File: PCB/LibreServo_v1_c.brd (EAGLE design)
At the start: 52.5 x 61.8 mm, 192 parts

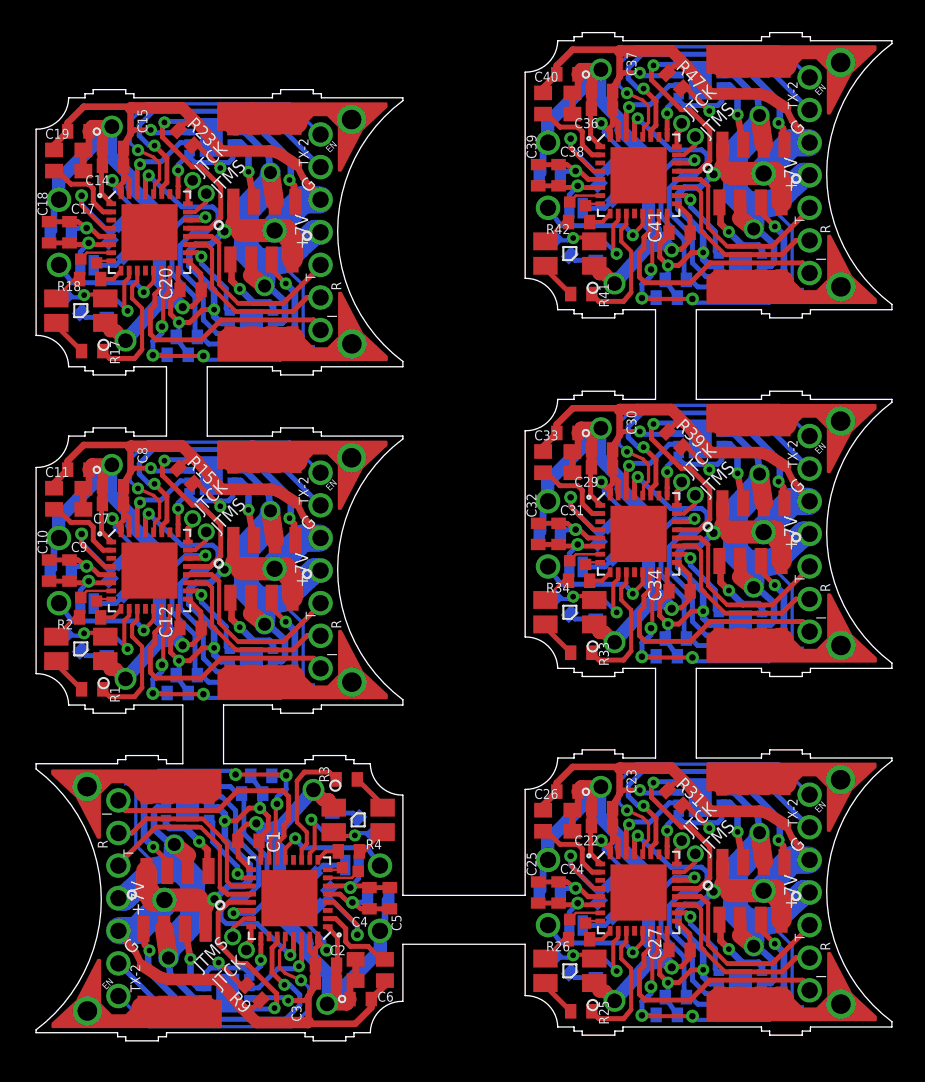
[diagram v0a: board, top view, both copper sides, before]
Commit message: LibreServo v1.c
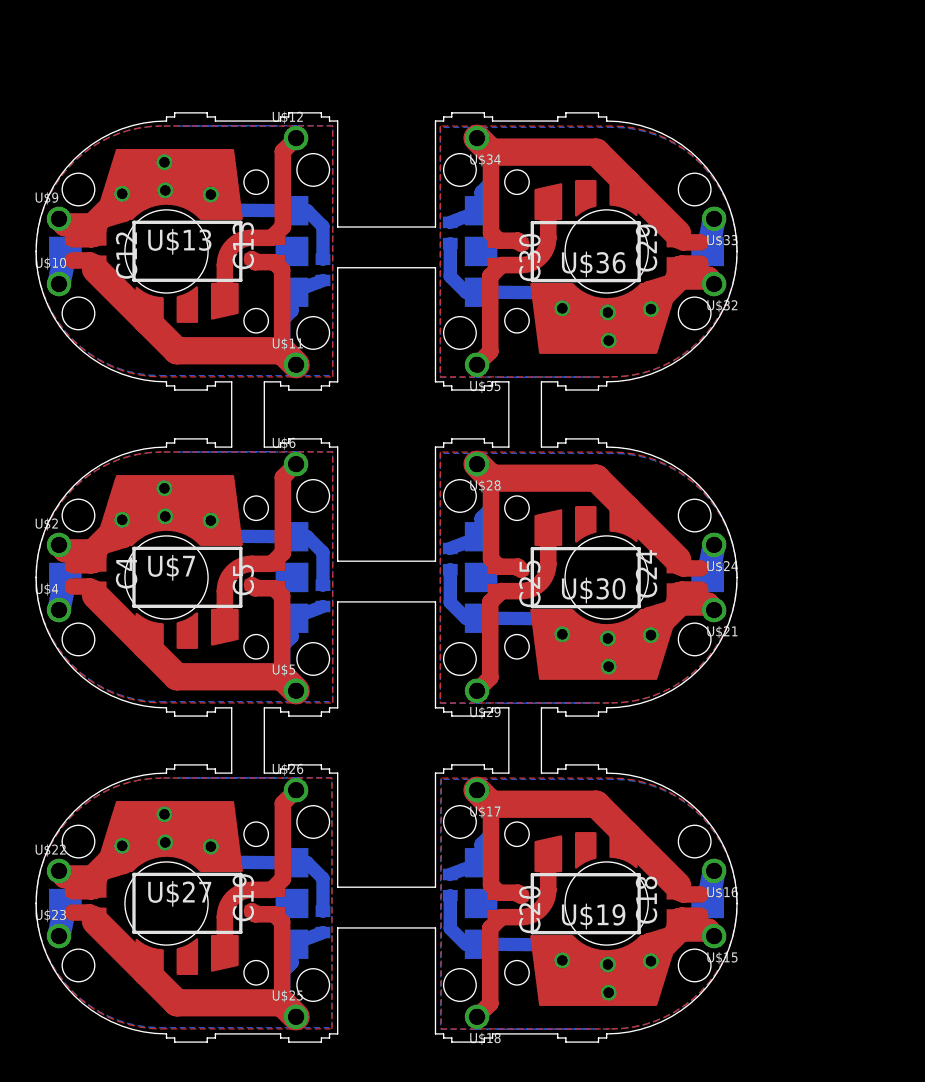
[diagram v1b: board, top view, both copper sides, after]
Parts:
- removed C31, C33, C34, C35, C36, C38, C40, C41, C42: 100nF, rcl:C0402
- removed C32, C39: 1uF, rcl:C0402
- removed C37: 4.7uF, rcl:C0402
- removed R1, R11, R12, R17, R18, R19, R2, R20, R25, R26, R27, R28, R3, R33, R34, R35, R36, R4, R41, R42, R43, R44, R5, R6: 160, rcl:R0402
- removed R10, R13, R15, R16, R21, R23, R24, R29, R31, R32, R37, R39, R40, R45, R47, R48, R7, R9: 10K, rcl:R0402
- removed R14, R22, R30, R38, R46, R8: 51K, rcl:R0402
- removed SJ1, SJ11, SJ3, SJ5, SJ7, SJ9: SOLDAR, SparkFun-Passives:SJ_2S
- removed SJ10, SJ12, SJ2, SJ4, SJ6, SJ8: NO-SOLDAR, SparkFun-Passives:SJ_2S-NO
- removed U$37, U$52, U$67, U$82: OSC-8MHz, Propio:OSC-2.5X2
- removed U$38, U$53, U$68, U$83: FERRITA, Propio:0402
- removed U$39, U$40, U$54, U$55, U$69, U$70, U$84, U$85: HEADER_1_MIN, Propio:HEADER_1_MIN
- removed U$41, U$56, U$71, U$86: HEADER_7_MIN, Propio:HEADER_7_MIN
- removed U$42, U$57, U$72, U$87: PAD_LIBRE_SERVO_V1_A, Propio:PAD_LIBRE_SERVO_V1_A
- removed U$43, U$58, U$73, U$88: PAD_LIBRE_SERVO_V1_B, Propio:PAD_LIBRE_SERVO_V1_B
- removed U$44, U$45, U$59, U$60, U$74, U$75, U$89, U$90: MICRO_PAD, Propio:MICRO_PAD
- removed U$46, U$61, U$76: STM32F302, Propio:QFN32
- removed U$47, U$48, U$62, U$63, U$77, U$78: FAN3227/3, Propio:MLP8
- removed U$49, U$50, U$64, U$65, U$79, U$80: FDS8858CZ, Propio:SO-8
- removed U$51, U$66, U$81: RGB_PLCC4, Propio:PLCC4
- C10: value 1uF -> 100nF
- C12, C13, C19, C20, C24, C29, C4: value 100nF -> 22uF; device rcl:C0402 -> Propio:0805_MIN
- C15, C23, C3: value 4.7uF -> 100nF
- C18, C25, C5: value 1uF -> 22uF; device rcl:C0402 -> Propio:0805_MIN
- C30, C8: value 4.7uF -> 22uF; device rcl:C0402 -> Propio:0805_MIN
- U$1, U$31: value STM32F302 -> MURATA_SV01; device Propio:QFN32 -> Propio:MURATA_SV01
- U$10, U$11, U$12, U$32, U$33: value FAN3227/3 -> HEADER_1_MIN; device Propio:MLP8 -> Propio:HEADER_1_MIN
- U$13, U$7: value FDS8858CZ -> NCP1117DT33G; device Propio:SO-8 -> Propio:SOT223_MOD
- U$14: value FDS8858CZ -> MURATA_SV01; device Propio:SO-8 -> Propio:MURATA_SV01
- U$17: value RGB_PLCC4 -> HEADER_1_MIN; device Propio:PLCC4 -> Propio:HEADER_1_MIN
- U$18, U$23: value HEADER_7_MIN -> HEADER_1_MIN; device Propio:HEADER_7_MIN -> Propio:HEADER_1_MIN
- U$19: value OSC-8MHz -> NCP1117DT33G; device Propio:OSC-2.5X2 -> Propio:SOT223_MOD
- U$2: value STM32F302 -> HEADER_1_MIN; device Propio:QFN32 -> Propio:HEADER_1_MIN
- U$20: value FERRITA -> MURATA_SV01; device Propio:0402 -> Propio:MURATA_SV01
- U$24, U$4: value PAD_LIBRE_SERVO_V1_A -> HEADER_1_MIN; device Propio:PAD_LIBRE_SERVO_V1_A -> Propio:HEADER_1_MIN
- U$25, U$28: value PAD_LIBRE_SERVO_V1_B -> HEADER_1_MIN; device Propio:PAD_LIBRE_SERVO_V1_B -> Propio:HEADER_1_MIN
- U$26, U$29: value MICRO_PAD -> HEADER_1_MIN; device Propio:MICRO_PAD -> Propio:HEADER_1_MIN
- U$27, U$30: value MICRO_PAD -> NCP1117DT33G; device Propio:MICRO_PAD -> Propio:SOT223_MOD
- U$3: value FAN3227/3 -> MURATA_SV01; device Propio:MLP8 -> Propio:MURATA_SV01
- U$34, U$35, U$6: value FDS8858CZ -> HEADER_1_MIN; device Propio:SO-8 -> Propio:HEADER_1_MIN
- U$36: value RGB_PLCC4 -> NCP1117DT33G; device Propio:PLCC4 -> Propio:SOT223_MOD
- U$5: value FERRITA -> HEADER_1_MIN; device Propio:0402 -> Propio:HEADER_1_MIN
- U$8: value RGB_PLCC4 -> MURATA_SV01; device Propio:PLCC4 -> Propio:MURATA_SV01
- U$9: value OSC-8MHz -> HEADER_1_MIN; device Propio:OSC-2.5X2 -> Propio:HEADER_1_MIN
- moved C14 57.9 mm to (40.7, 8.40), turned to 90 degrees
- moved C18 56.4 mm to (39.4, 8.45), turned to 90 degrees
- moved C15 52.8 mm to (29.8, 8.31), turned to 270 degrees
- moved U$9 49.9 mm to (1.40, 50.5), turned to 0 degrees
- moved C6 49.2 mm to (2.26, 48.6), turned to 270 degrees
- moved C19 48.8 mm to (14.6, 8.59), turned to 90 degrees
- moved C17 45.1 mm to (17.6, 7.37), flipped to the bottom
- moved C27 43.8 mm to (29.8, 48.3), turned to 270 degrees
- moved C28 42.6 mm to (25.4, 49.6), turned to 90 degrees
- moved C20 42.2 mm to (28.4, 8.41), turned to 270 degrees
- moved U$12 41.3 mm to (15.9, 55.5), flipped to the top
- moved C21 41.1 mm to (40.7, 28.4), flipped to the top, turned to 90 degrees
- moved U$19 40.3 mm to (33.7, 8.49), turned to 180 degrees
- moved U$21 40.2 mm to (41.6, 26.5), turned to 180 degrees
- moved U$11 38.8 mm to (15.9, 41.5), flipped to the top
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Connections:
- removed net EN_Q1: R9.2, U$1.25, U$11.P$1, U$11.P$8
- removed net EN_Q10: R40.1, U$61.22, U$63.P$1, U$63.P$8
- removed net EN_Q11: R47.2, U$76.25, U$77.P$1, U$77.P$8
- removed net EN_Q12: R48.1, U$76.22, U$78.P$1, U$78.P$8
- removed net EN_Q2: R10.1, U$1.22, U$12.P$1, U$12.P$8
- removed net EN_Q3: R15.2, U$2.25, U$3.P$1, U$3.P$8
- removed net EN_Q4: R16.1, U$10.P$1, U$10.P$8, U$2.22
- removed net EN_Q5: R23.2, U$31.25, U$32.P$1, U$32.P$8
- removed net EN_Q6: R24.1, U$31.22, U$33.P$1, U$33.P$8
- removed net EN_Q7: R31.2, U$46.25, U$47.P$1, U$47.P$8
- removed net EN_Q8: R32.1, U$46.22, U$48.P$1, U$48.P$8
- removed net EN_Q9: R39.2, U$61.25, U$62.P$1, U$62.P$8
- removed net EN_SERIAL_1: U$1.28, U$18.P$1
- removed net EN_SERIAL_2: U$2.28, U$23.P$1
- removed net EN_SERIAL_3: U$31.28, U$41.P$1
- removed net EN_SERIAL_4: U$46.28, U$56.P$1
- removed net EN_SERIAL_5: U$61.28, U$71.P$1
- removed net EN_SERIAL_6: U$76.28, U$86.P$1
- removed net GNDA: C4.2, C5.2, SJ1.2, U$1.6
- removed net GNDA1: C10.2, C9.2, SJ3.2, U$2.6
- removed net GNDA2: C17.2, C18.2, SJ5.2, U$31.6
- removed net GNDA3: C24.2, C25.2, SJ7.2, U$46.6
- removed net GNDA4: C31.2, C32.2, SJ9.2, U$61.6
- removed net GNDA5: C38.2, C39.2, SJ11.2, U$76.6
- removed net GND_1: C1.1, C16.2, C2.2, C3.1, C6.2, R10.2, R7.2, R9.1, SJ1.1, SJ2.1, U$1.16, U$1.31, U$1.32, U$11.P$3, U$12.P$3, U$18.P$3, U$6.P$1, U$7.P$1, U$9.P$2
- removed net GND_2: C11.2, C12.1, C13.2, C7.2, C8.1, R13.2, R15.1, R16.2, SJ3.1, SJ4.1, U$10.P$3, U$13.P$1, U$14.P$1, U$19.P$2, U$2.16, U$2.31, U$2.32, U$23.P$3, U$3.P$3
- removed net GND_3: C14.2, C15.1, C19.2, C20.1, C21.2, R21.2, R23.1, R24.2, SJ5.1, SJ6.1, U$31.16, U$31.31, U$31.32, U$32.P$3, U$33.P$3, U$34.P$1, U$35.P$1, U$37.P$2, U$41.P$3
- removed net GND_4: C22.2, C23.1, C26.2, C27.1, C28.2, R29.2, R31.1, R32.2, SJ7.1, SJ8.1, U$46.16, U$46.31, U$46.32, U$47.P$3, U$48.P$3, U$49.P$1, U$50.P$1, U$52.P$2, U$56.P$3
- removed net GND_5: C29.2, C30.1, C33.2, C34.1, C35.2, R37.2, R39.1, R40.2, SJ10.1, SJ9.1, U$61.16, U$61.31, U$61.32, U$62.P$3, U$63.P$3, U$64.P$1, U$65.P$1, U$67.P$2, U$71.P$3
- removed net GND_6: C36.2, C37.1, C40.2, C41.1, C42.2, R45.2, R47.1, R48.2, SJ11.1, SJ12.1, U$76.16, U$76.31, U$76.32, U$77.P$3, U$78.P$3, U$79.P$1, U$80.P$1, U$82.P$2, U$86.P$3
- removed net JTCK: U$1.24
- removed net JTCK1: U$2.24
- removed net JTCK2: U$31.24
- removed net JTCK3: U$46.24
- removed net JTCK4: U$61.24
- removed net JTCK5: U$76.24
- removed net JTMS: U$1.23
- removed net JTMS1: U$2.23
- removed net JTMS2: U$31.23
- removed net JTMS3: U$46.23
- removed net JTMS4: U$61.23
- removed net JTMS5: U$76.23
- removed net LED_BLUE: R3.2, U$1.11
- removed net LED_BLUE1: R1.2, U$2.11
- removed net LED_BLUE2: R17.2, U$31.11
- removed net LED_BLUE3: R25.2, U$46.11
- removed net LED_BLUE4: R33.2, U$61.11
- removed net LED_BLUE5: R41.2, U$76.11
- removed net LED_GREEN: R4.2, U$1.9
- removed net LED_GREEN1: R2.2, U$2.9
- removed net LED_GREEN2: R18.2, U$31.9
- removed net LED_GREEN3: R26.2, U$46.9
- removed net LED_GREEN4: R34.2, U$61.9
- removed net LED_GREEN5: R42.2, U$76.9
- removed net LED_RED: R5.2, U$1.10
- removed net LED_RED1: R11.2, U$2.10
- removed net LED_RED2: R19.2, U$31.10
- removed net LED_RED3: R27.2, U$46.10
- removed net LED_RED4: R35.2, U$61.10
- removed net LED_RED5: R43.2, U$76.10
- removed net N$1: R3.1, U$8.P$2
- removed net N$10: U$11.P$7, U$6.P$2
- removed net N$11: U$13.P$4, U$3.P$5
- removed net N$12: U$10.P$7, U$14.P$2
- removed net N$13: U$10.P$5, U$14.P$4
- removed net N$14: U$11.P$5, U$6.P$4
- removed net N$15: U$12.P$7, U$7.P$2
- removed net N$16: U$13.P$5, U$13.P$6, U$13.P$7, U$13.P$8, U$25.P$1, U$25.P$2
- removed net N$17: U$14.P$5, U$14.P$6, U$14.P$7, U$14.P$8, U$24.P$1, U$24.P$2
- removed net N$18: U$12.P$5, U$7.P$4
- removed net N$19: U$28.P$1, U$28.P$2, U$6.P$5, U$6.P$6, U$6.P$7, U$6.P$8
- removed net N$2: R4.1, U$8.P$3
- removed net N$20: R1.1, U$17.P$2
- removed net N$21: R2.1, U$17.P$3
- removed net N$22: R11.1, R12.2
- removed net N$23: R12.1, U$17.P$4
- removed net N$24: U$2.7, U$26.P$1
- removed net N$25: U$2.8, U$27.P$1
- removed net N$26: U$4.P$1, U$4.P$2, U$7.P$5, U$7.P$6, U$7.P$7, U$7.P$8
- removed net N$27: U$31.2, U$37.P$3
- removed net N$28: U$32.P$7, U$34.P$2
- removed net N$29: U$32.P$5, U$34.P$4
- removed net N$3: R6.1, U$8.P$4
- removed net N$30: U$33.P$7, U$35.P$2
- removed net N$31: U$33.P$5, U$35.P$4
- removed net N$32: U$34.P$5, U$34.P$6, U$34.P$7, U$34.P$8, U$43.P$1, U$43.P$2
- removed net N$33: U$35.P$5, U$35.P$6, U$35.P$7, U$35.P$8, U$42.P$1, U$42.P$2
- removed net N$34: R17.1, U$36.P$2
- removed net N$35: R18.1, U$36.P$3
- removed net N$36: R19.1, R20.2
- removed net N$37: R20.1, U$36.P$4
- removed net N$38: U$31.7, U$44.P$1
- removed net N$39: U$31.8, U$45.P$1
- removed net N$4: U$1.7, U$29.P$1
- removed net N$40: U$46.2, U$52.P$3
- removed net N$41: U$47.P$7, U$49.P$2
- removed net N$42: U$47.P$5, U$49.P$4
- removed net N$43: U$48.P$7, U$50.P$2
- removed net N$44: U$48.P$5, U$50.P$4
- removed net N$45: U$49.P$5, U$49.P$6, U$49.P$7, U$49.P$8, U$58.P$1, U$58.P$2
- removed net N$46: U$50.P$5, U$50.P$6, U$50.P$7, U$50.P$8, U$57.P$1, U$57.P$2
- removed net N$47: R25.1, U$51.P$2
- removed net N$48: R26.1, U$51.P$3
- removed net N$49: R27.1, R28.2
- removed net N$5: U$1.2, U$9.P$3
- removed net N$50: R28.1, U$51.P$4
- removed net N$51: U$46.7, U$59.P$1
- removed net N$52: U$46.8, U$60.P$1
- removed net N$53: U$61.2, U$67.P$3
- removed net N$54: U$62.P$7, U$64.P$2
- removed net N$55: U$62.P$5, U$64.P$4
- removed net N$56: U$63.P$7, U$65.P$2
- removed net N$57: U$63.P$5, U$65.P$4
- removed net N$58: U$64.P$5, U$64.P$6, U$64.P$7, U$64.P$8, U$73.P$1, U$73.P$2
- removed net N$59: U$65.P$5, U$65.P$6, U$65.P$7, U$65.P$8, U$72.P$1, U$72.P$2
- removed net N$6: R5.1, R6.2
- removed net N$60: R33.1, U$66.P$2
- removed net N$61: R34.1, U$66.P$3
- removed net N$62: R35.1, R36.2
- removed net N$63: R36.1, U$66.P$4
- removed net N$64: U$61.7, U$74.P$1
- removed net N$65: U$61.8, U$75.P$1
- removed net N$66: U$76.2, U$82.P$3
- removed net N$67: U$77.P$7, U$79.P$2
- removed net N$68: U$77.P$5, U$79.P$4
- removed net N$69: U$78.P$7, U$80.P$2
- removed net N$7: U$1.8, U$30.P$1
- removed net N$70: U$78.P$5, U$80.P$4
- removed net N$71: U$79.P$5, U$79.P$6, U$79.P$7, U$79.P$8, U$88.P$1, U$88.P$2
- removed net N$72: U$80.P$5, U$80.P$6, U$80.P$7, U$80.P$8, U$87.P$1, U$87.P$2
- removed net N$73: R41.1, U$81.P$2
- removed net N$74: R42.1, U$81.P$3
- removed net N$75: R43.1, R44.2
- removed net N$76: R44.1, U$81.P$4
- removed net N$77: U$76.7, U$89.P$1
- removed net N$78: U$76.8, U$90.P$1
- removed net N$8: U$19.P$3, U$2.2
- removed net N$9: U$13.P$2, U$3.P$7
- removed net NRST: C16.1, SJ2.2, U$1.4
- removed net NRST1: C13.1, SJ4.2, U$2.4
- removed net NRST2: C21.1, SJ6.2, U$31.4
- removed net NRST3: C28.1, SJ8.2, U$46.4
- removed net NRST4: C35.1, SJ10.2, U$61.4
- removed net NRST5: C42.1, SJ12.2, U$76.4
- removed net Q1_INA_N: U$1.30, U$11.P$2
- removed net Q1_INA_N1: U$2.30, U$3.P$2
- removed net Q1_INA_N2: U$31.30, U$32.P$2
- removed net Q1_INA_N3: U$46.30, U$47.P$2
- removed net Q1_INA_N4: U$61.30, U$62.P$2
- removed net Q1_INA_N5: U$76.30, U$77.P$2
- removed net Q2_INA_N: U$1.29, U$12.P$2
- removed net Q2_INA_N1: U$10.P$2, U$2.29
- removed net Q2_INA_N2: U$31.29, U$33.P$2
- removed net Q2_INA_N3: U$46.29, U$48.P$2
- removed net Q2_INA_N4: U$61.29, U$63.P$2
- removed net Q2_INA_N5: U$76.29, U$78.P$2
- removed net RX_1: U$1.19, U$18.P$6
- removed net RX_2: U$2.19, U$23.P$6
- removed net RX_3: U$31.19, U$41.P$6
- removed net RX_4: U$46.19, U$56.P$6
- removed net RX_5: U$61.19, U$71.P$6
- removed net RX_6: U$76.19, U$86.P$6
- removed net TIM1_CH1: U$1.18, U$12.P$4
- removed net TIM1_CH10: U$61.18, U$63.P$4
- removed net TIM1_CH11: U$76.21, U$77.P$4
- removed net TIM1_CH12: U$76.18, U$78.P$4
- removed net TIM1_CH2: U$2.21, U$3.P$4
- removed net TIM1_CH3: U$10.P$4, U$2.18
- removed net TIM1_CH4: U$1.21, U$11.P$4
- removed net TIM1_CH5: U$31.21, U$32.P$4
- removed net TIM1_CH6: U$31.18, U$33.P$4
- removed net TIM1_CH7: U$46.21, U$47.P$4
- removed net TIM1_CH8: U$46.18, U$48.P$4
- removed net TIM1_CH9: U$61.21, U$62.P$4
- removed net TX_1: U$1.20, U$18.P$5
- removed net TX_2: U$2.20, U$23.P$5
- removed net TX_3: U$31.20, U$41.P$5
- removed net TX_4: U$46.20, U$56.P$5
- removed net TX_5: U$61.20, U$71.P$5
- removed net TX_6: U$76.20, U$86.P$5
- removed net USART2_RX_1: U$1.27, U$18.P$2
- removed net USART2_RX_2: U$2.27, U$23.P$2
- removed net USART2_RX_3: U$31.27, U$41.P$2
- removed net USART2_RX_4: U$46.27, U$56.P$2
- removed net USART2_RX_5: U$61.27, U$71.P$2
- removed net USART2_RX_6: U$76.27, U$86.P$2
- removed net VBAT: R7.1, R8.2, U$1.15
- removed net VBAT1: R13.1, R14.2, U$2.15
- removed net VBAT2: R21.1, R22.2, U$31.15
- removed net VBAT3: R29.1, R30.2, U$46.15
- removed net VBAT4: R37.1, R38.2, U$61.15
- removed net VBAT5: R45.1, R46.2, U$76.15
- removed net VDD: C4.1, C5.1, U$1.5, U$5.2
- removed net VDD1: C10.1, C9.1, U$2.5, U$20.2
- removed net VDD2: C17.1, C18.1, U$31.5, U$38.2
- removed net VDD3: C24.1, C25.1, U$46.5, U$53.2
- removed net VDD4: C31.1, C32.1, U$61.5, U$68.2
- removed net VDD5: C38.1, C39.1, U$76.5, U$83.2
- removed net V_CORRIENTE_1: U$1.14, U$18.P$7
- removed net V_CORRIENTE_2: U$2.14, U$23.P$7
- removed net V_CORRIENTE_3: U$31.14, U$41.P$7
- removed net V_CORRIENTE_4: U$46.14, U$56.P$7
- removed net V_CORRIENTE_5: U$61.14, U$71.P$7
- removed net V_CORRIENTE_6: U$76.14, U$86.P$7
- new net GND1: C1.2, C2.1, C3.2, C4.2, C5.1, U$1.P$3, U$5.P$1, U$7.P$1
- new net GND2: C11.2, C12.2, C13.1, C6.2, C7.1, U$11.P$1, U$13.P$1, U$8.P$3
- new net GND3: C10.2, C17.2, C19.1, C8.2, C9.1, U$25.P$1, U$27.P$1, U$3.P$3
- new net GND4: C14.2, C15.1, C16.2, C18.2, C20.1, U$14.P$3, U$17.P$1, U$19.P$1
- new net GND5: C21.2, C22.1, C23.2, C24.2, C25.1, U$20.P$3, U$28.P$1, U$30.P$1
- new net GND6: C26.2, C27.1, C28.2, C29.2, C30.1, U$31.P$3, U$34.P$1, U$36.P$1
- net +3V3_1: now also C1.1, C3.1, C4.1, U$1.P$1, U$2.P$1, U$7.P$4; no longer C1.2, C2.1, C3.2, C6.1, U$1.1, U$1.17, U$16.P$1, U$5.1, U$8.P$1, U$9.P$1, U$9.P$4
- net +3V3_2: now also C12.1, C6.1, U$13.P$4, U$8.P$1, U$9.P$1; no longer C12.2, C7.1, C8.2, U$17.P$1, U$19.P$1, U$19.P$4, U$2.1, U$2.17, U$20.1, U$22.P$1
- net +3V3_3: now also C10.1, C17.1, C8.1, U$22.P$1, U$27.P$4, U$3.P$1; no longer C14.1, C15.2, C19.1, C20.2, U$31.1, U$31.17, U$36.P$1, U$37.P$1, U$37.P$4, U$38.1, U$40.P$1
- net +3V3_4: now also C14.1, C16.1, C18.1, U$14.P$1, U$15.P$1, U$19.P$4; no longer C22.1, C23.2, C26.1, C27.2, U$46.1, U$46.17, U$51.P$1, U$52.P$1, U$52.P$4, U$53.1, U$55.P$1
- net +3V3_5: now also C21.1, C23.1, C24.1, U$20.P$1, U$21.P$1, U$30.P$4; no longer C29.1, C30.2, C33.1, C34.2, U$61.1, U$61.17, U$66.P$1, U$67.P$1, U$67.P$4, U$68.1, U$70.P$1
- net +3V3_6: now also C26.1, C28.1, C29.1, U$31.P$1, U$32.P$1, U$36.P$4; no longer C36.1, C37.2, C40.1, C41.2, U$76.1, U$76.17, U$81.P$1, U$82.P$1, U$82.P$4, U$83.1, U$85.P$1
- net +7V_1: now also C2.2, C5.2, U$6.P$1; no longer R8.1, U$11.P$6, U$12.P$6, U$18.P$4, U$6.P$3
- net +7V_2: now also C13.2, C7.2, U$12.P$1; no longer R14.1, U$10.P$6, U$14.P$3, U$23.P$4, U$3.P$6
- net +7V_3: now also C19.2, C9.2, U$26.P$1, U$27.P$3; no longer R22.1, U$32.P$6, U$33.P$6, U$34.P$3, U$35.P$3, U$41.P$4
- net +7V_4: now also C15.2, C20.2, U$18.P$1, U$19.P$3; no longer R30.1, U$47.P$6, U$48.P$6, U$49.P$3, U$50.P$3, U$56.P$4
- net +7V_5: now also C22.2, C25.2, U$29.P$1, U$30.P$3; no longer R38.1, U$62.P$6, U$63.P$6, U$64.P$3, U$65.P$3, U$71.P$4
- net +7V_6: now also C27.2, C30.2, U$35.P$1, U$36.P$3; no longer R46.1, U$77.P$6, U$78.P$6, U$79.P$3, U$80.P$3, U$86.P$4
- net V_POT_1: now also U$1.P$4, U$4.P$1; no longer U$1.13, U$15.P$1
- net V_POT_2: now also U$10.P$1, U$8.P$4; no longer U$2.13, U$21.P$1
- net V_POT_3: now also U$23.P$1, U$3.P$4; no longer U$31.13, U$39.P$1
- net V_POT_4: now also U$14.P$4, U$16.P$1; no longer U$46.13, U$54.P$1
- net V_POT_5: now also U$20.P$4, U$24.P$1; no longer U$61.13, U$69.P$1
- net V_POT_6: now also U$31.P$4, U$33.P$1; no longer U$76.13, U$84.P$1
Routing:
- net GND_6: track 69.9 -> 0.00 mm, vias 6 -> 0
- net GND_4: track 69.9 -> 0.00 mm, vias 6 -> 0
- net GND_3: track 69.9 -> 0.00 mm, vias 6 -> 0
- net GND_2: track 69.9 -> 0.00 mm, vias 6 -> 0
- net GND_5: track 69.9 -> 0.00 mm, vias 6 -> 0
- net GND_1: track 69.9 -> 0.00 mm, vias 6 -> 0
- net GND2: track 0.00 -> 30.6 mm
- net GND5: track 0.00 -> 30.6 mm
- net GND1: track 0.00 -> 30.6 mm
- net GND6: track 0.00 -> 30.6 mm
- net GND3: track 0.00 -> 30.6 mm
- net GND4: track 0.00 -> 30.6 mm
- net EN_SERIAL_6: track 18.5 -> 0.00 mm, vias 1 -> 0
- net EN_SERIAL_5: track 18.5 -> 0.00 mm, vias 1 -> 0
- net EN_SERIAL_3: track 18.5 -> 0.00 mm, vias 1 -> 0
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- added copper zone on layer 16, net +3V3_1
- added copper zone on layer 16, net +3V3_2
- added copper zone on layer 16, net +3V3_3
- added copper zone on layer 16, net +3V3_4
- added copper zone on layer 16, net +3V3_5
- added copper zone on layer 16, net +3V3_6
- added copper zone on layer 1, net GND1
- added copper zone on layer 1, net GND2
- added copper zone on layer 1, net GND3
- added copper zone on layer 1, net GND4
- added copper zone on layer 1, net GND5
- added copper zone on layer 1, net GND6
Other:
- board size 52.5 x 61.8 mm -> 43 x 57 mm
- board text added: "+3V3"
- board text added: "C10"
- board text added: "C17"
- board text added: "C8"
- board text added: "C9"
- board text added: "LibreServo v1.c"
- board text removed: "EN"
- board text removed: "EN-S"
- board text removed: "G"
- board text removed: "I"
- board text removed: "JTCK"
- board text removed: "JTMS"
- board text removed: "R"
- board text removed: "RX"
- board text removed: "T"
- board text removed: "TX"
- board text removed: "TX-2"
